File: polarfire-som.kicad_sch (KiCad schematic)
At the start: 12 parts

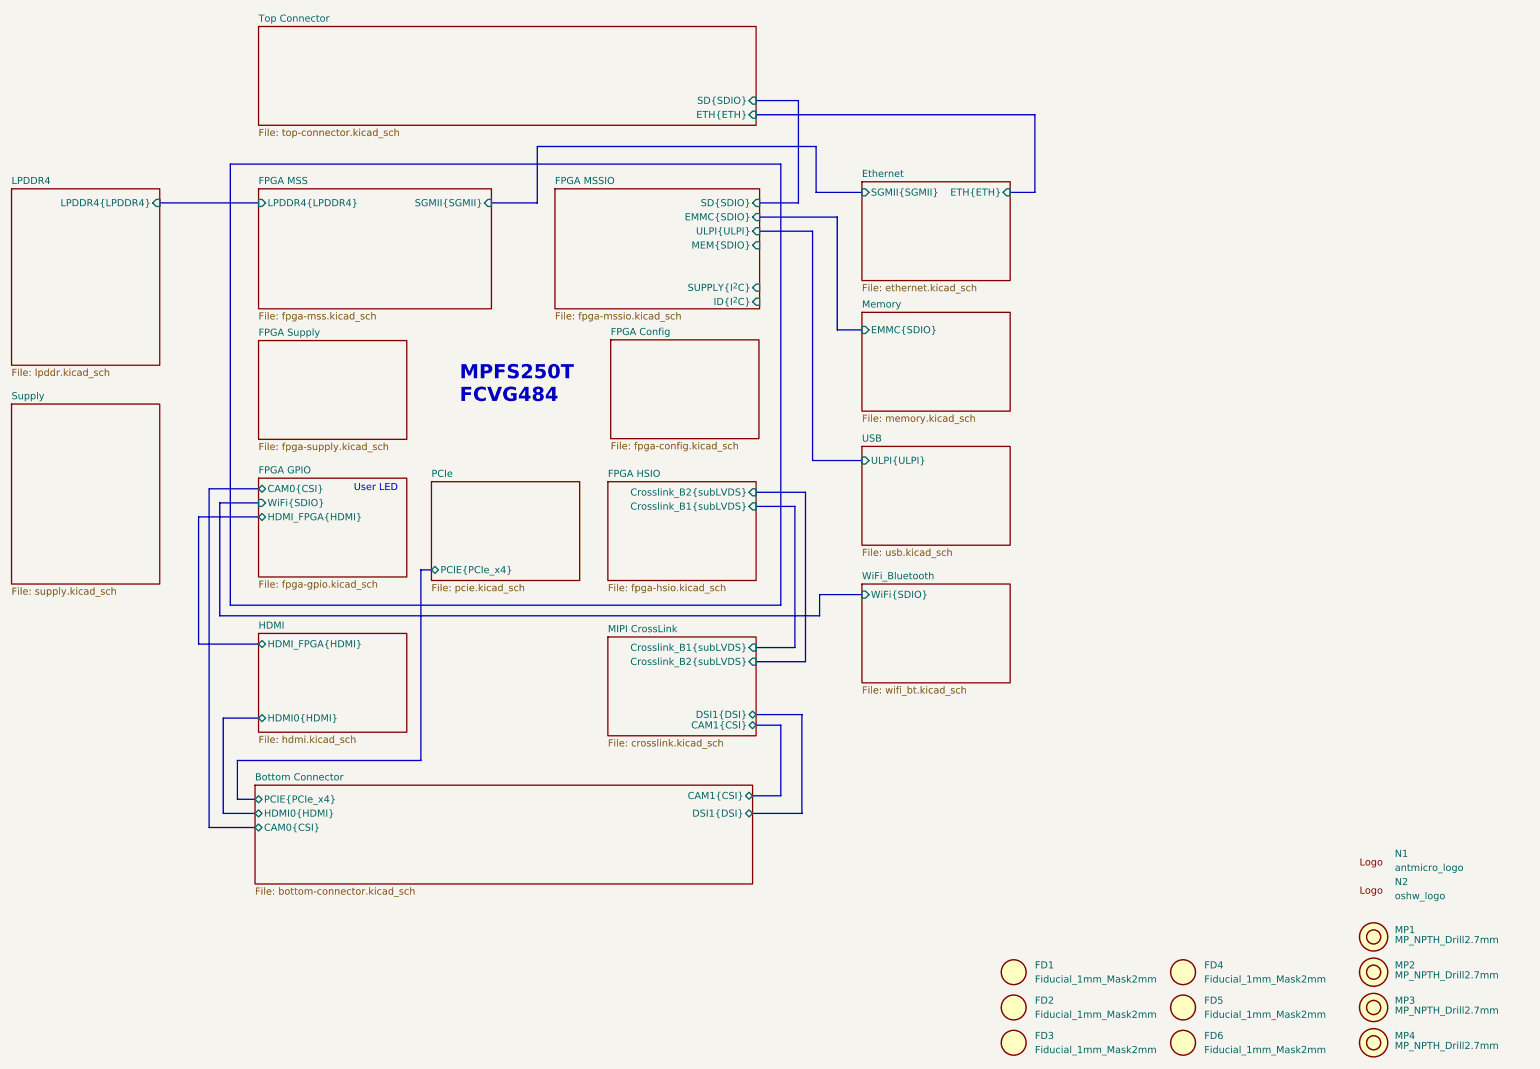
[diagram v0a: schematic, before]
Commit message: [#57505] Finish defining buses
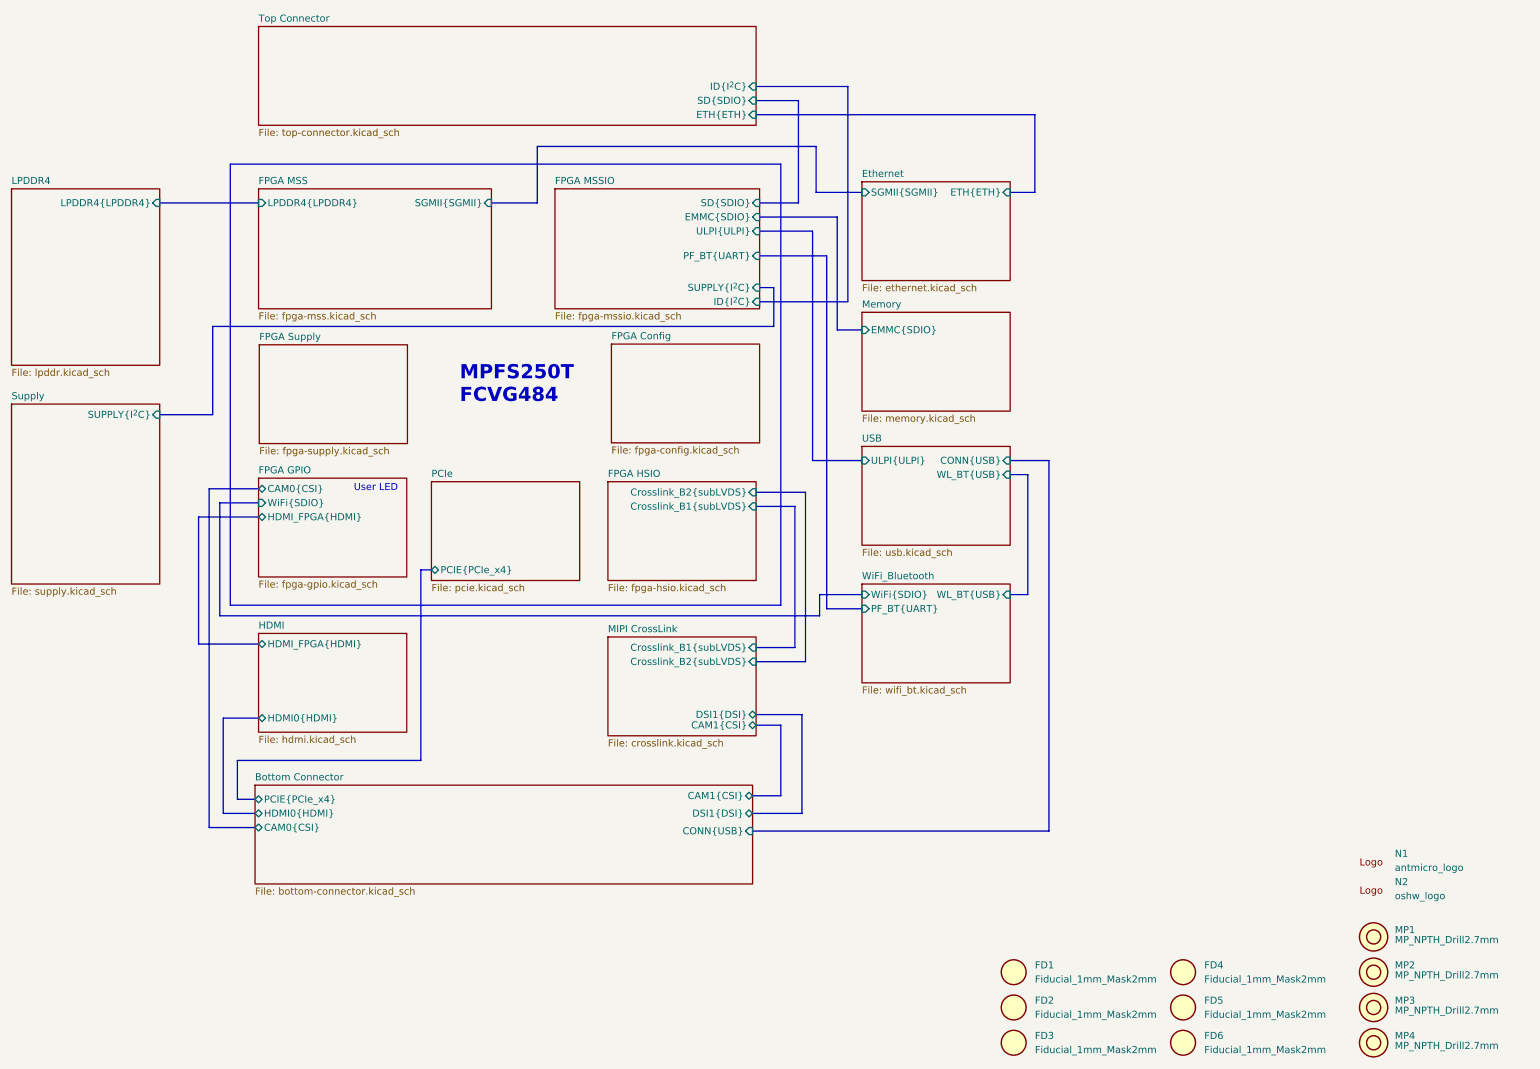
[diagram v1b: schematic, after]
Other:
- sheet Bottom Connector ports: added CONN{USB}; removed none
- sheet FPGA MSSIO ports: added PF_BT{UART}; removed MEM{SDIO}
- sheet Supply ports: added SUPPLY{I^{2}C}; removed none
- sheet Top Connector ports: added ID{I^{2}C}; removed none
- sheet USB ports: added CONN{USB}, WL_BT{USB}; removed none
- sheet WiFi_Bluetooth ports: added PF_BT{UART}, WL_BT{USB}; removed none
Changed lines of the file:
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@@
+    (stroke (width 0) (type default))
+  )
+  (bus (pts (xy 262.89 106.68) (xy 265.43 106.68))
     (stroke (width 0) (type default))
   )
@@
     (stroke (width 0) (type default))
   )
+  (bus (pts (xy 278.765 70.485) (xy 278.765 109.22))
+    (stroke (width 0) (type default))
+  )
   (bus (pts (xy 165.735 165.735) (xy 273.685 165.735))
     (stroke (width 0) (type default))
   )
+  (bus (pts (xy 311.15 140.335) (xy 311.15 161.925))
+    (stroke (width 0) (type default))
+  )
   (polyline (pts (xy 266.7 84.455) (xy 266.7 163.83))
     (stroke (width 0) (type default))
@@
     (stroke (width 0) (type default))
   )
+  (bus (pts (xy 265.43 106.68) (xy 265.43 113.665))
+    (stroke (width 0) (type default))
+  )
   (bus (pts (xy 201.93 157.48) (xy 203.835 157.48))
     (stroke (width 0) (type default))
@@
     (stroke (width 0) (type default))
   )
+  (bus (pts (xy 262.89 100.965) (xy 274.955 100.965))
+    (stroke (width 0) (type default))
+  )
   (bus (pts (xy 161.925 170.815) (xy 161.925 147.955))
     (stroke (width 0) (type default))
@@
     (stroke (width 0) (type default))
   )
+  (bus (pts (xy 311.15 161.925) (xy 307.975 161.925))
+    (stroke (width 0) (type default))
+  )
+  (bus (pts (xy 274.955 164.465) (xy 281.305 164.465))
+    (stroke (width 0) (type default))
+  )
+  (bus (pts (xy 307.975 140.335) (xy 311.15 140.335))
+    (stroke (width 0) (type default))
+  )
   (bus (pts (xy 312.42 75.565) (xy 312.42 89.535))
     (stroke (width 0) (type default))
   )
+  (bus (pts (xy 274.955 100.965) (xy 274.955 164.465))
+    (stroke (width 0) (type default))
+  )
+  (bus (pts (xy 262.255 70.485) (xy 278.765 70.485))
+    (stroke (width 0) (type default))
+  )
   (bus (pts (xy 163.83 142.875) (xy 172.72 142.875))
     (stroke (width 0) (type default))
   )
+  (bus (pts (xy 265.43 113.665) (xy 164.465 113.665))
+    (stroke (width 0) (type default))
+  )
   (bus (pts (xy 172.72 145.415) (xy 165.735 145.415))
     (stroke (width 0) (type default))
@@
     (stroke (width 0) (type default))
   )
+  (bus (pts (xy 314.96 204.47) (xy 314.96 137.795))
+    (stroke (width 0) (type default))
+  )
+  (bus (pts (xy 164.465 113.665) (xy 164.465 129.54))
+    (stroke (width 0) (type default))
+  )
   (bus (pts (xy 273.685 165.735) (xy 273.685 161.925))
     (stroke (width 0) (type default))
@@
     (stroke (width 0) (type default))
   )
+  (bus (pts (xy 164.465 129.54) (xy 154.94 129.54))
+    (stroke (width 0) (type default))
+  )
   (bus (pts (xy 201.93 157.48) (xy 201.93 191.77))
     (stroke (width 0) (type default))
@@
     (stroke (width 0) (type default))
   )
+  (bus (pts (xy 261.62 204.47) (xy 314.96 204.47))
+    (stroke (width 0) (type default))
+  )
+  (bus (pts (xy 314.96 137.795) (xy 307.975 137.795))
+    (stroke (width 0) (type default))
+  )
   (bus (pts (xy 222.885 81.28) (xy 273.05 81.28))
     (stroke (width 0) (type default))
   )
   (bus (pts (xy 271.145 173.99) (xy 262.255 173.99))
+    (stroke (width 0) (type default))
+  )
+  (bus (pts (xy 278.765 109.22) (xy 262.89 109.22))
     (stroke (width 0) (type default))
   )
@@
       (effects (font (size 1.27 1.27)) (justify left))
     )
+    (pin "WL_BT{USB}" input (at 307.975 161.925 0)
+      (effects (font (size 1.27 1.27)) (justify right))
+    )
+    (pin "PF_BT{UART}" input (at 281.305 164.465 180)
+      (effects (font (size 1.27 1.27)) (justify left))
+    )
     (instances
       (project "polarfire-som"
@@
     )
   )
-  (sheet (at 172.72 116.205) (size 26.67 17.78) (fields_autoplaced)
+  (sheet (at 172.847 116.967) (size 26.67 17.78) (fields_autoplaced)
     (stroke (width 0.1524) (type solid))
     (fill (color 0 0 0 0.0000))
-    (property "Sheetname" "FPGA Supply" (at 172.72 115.4934 0)
+    (property "Sheetname" "FPGA Supply" (at 172.847 116.2554 0)
       (effects (font (size 1.27 1.27)) (justify left bottom))
     )
-    (property "Sheetfile" "fpga-supply.kicad_sch" (at 172.72 134.5696 0)
+    (property "Sheetfile" "fpga-supply.kicad_sch" (at 172.847 135.3316 0)
       (effects (font (size 1.27 1.27)) (justify left top))
     )
@@
       (effects (font (size 1.27 1.27)) (justify left top))
     )
+    (pin "SUPPLY{I^{2}C}" input (at 154.94 129.54 0)
+      (effects (font (size 1.27 1.27)) (justify right))
+    )
     (instances
       (project "polarfire-som"
@@
       (effects (font (size 1.27 1.27)) (justify right))
     )
+    (pin "CONN{USB}" input (at 261.62 204.47 0)
+      (effects (font (size 1.27 1.27)) (justify right))
+    )
     (instances
       (project "polarfire-som"
@@
       (effects (font (size 1.27 1.27)) (justify left))
     )
+    (pin "WL_BT{USB}" input (at 307.975 140.335 0)
+      (effects (font (size 1.27 1.27)) (justify right))
+    )
+    (pin "CONN{USB}" input (at 307.975 137.795 0)
+      (effects (font (size 1.27 1.27)) (justify right))
+    )
     (instances
       (project "polarfire-som"
@@
     )
   )
-  (sheet (at 236.093 116.078) (size 26.67 17.78) (fields_autoplaced)
+  (sheet (at 236.22 116.84) (size 26.67 17.78) (fields_autoplaced)
     (stroke (width 0.1524) (type solid))
     (fill (color 0 0 0 0.0000))
-    (property "Sheetname" "FPGA Config" (at 236.093 115.3664 0)
+    (property "Sheetname" "FPGA Config" (at 236.22 116.1284 0)
       (effects (font (size 1.27 1.27)) (justify left bottom))
     )
-    (property "Sheetfile" "fpga-config.kicad_sch" (at 236.093 134.4426 0)
+    (property "Sheetfile" "fpga-config.kicad_sch" (at 236.22 135.2046 0)
       (effects (font (size 1.27 1.27)) (justify left top))
     )
@@
       (effects (font (size 1.27 1.27)) (justify right))
     )
+    (pin "ID{I^{2}C}" input (at 262.255 70.485 0)
+      (effects (font (size 1.27 1.27)) (justify right))
+    )
     (instances
       (project "polarfire-som"
@@
       (effects (font (size 1.27 1.27)) (justify right))
     )
-    (pin "MEM{SDIO}" input (at 262.89 99.06 0)
-      (effects (font (size 1.27 1.27)) (justify right))
-    )
     (pin "SUPPLY{I^{2}C}" input (at 262.89 106.68 0)
       (effects (font (size 1.27 1.27)) (justify right))
@@
       (effects (font (size 1.27 1.27)) (justify right))
     )
+    (pin "PF_BT{UART}" input (at 262.89 100.965 0)
+      (effects (font (size 1.27 1.27)) (justify right))
+    )
